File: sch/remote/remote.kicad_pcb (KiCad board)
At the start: 2 copper layers, 24 parts, among them J1 swd, J2 power_sw, J3 USB_A, Q1 DTD114E, U1 STM32F103C8Tx_usb, U2 XC6206-33, U3 TSOP17xx, Y1 8M

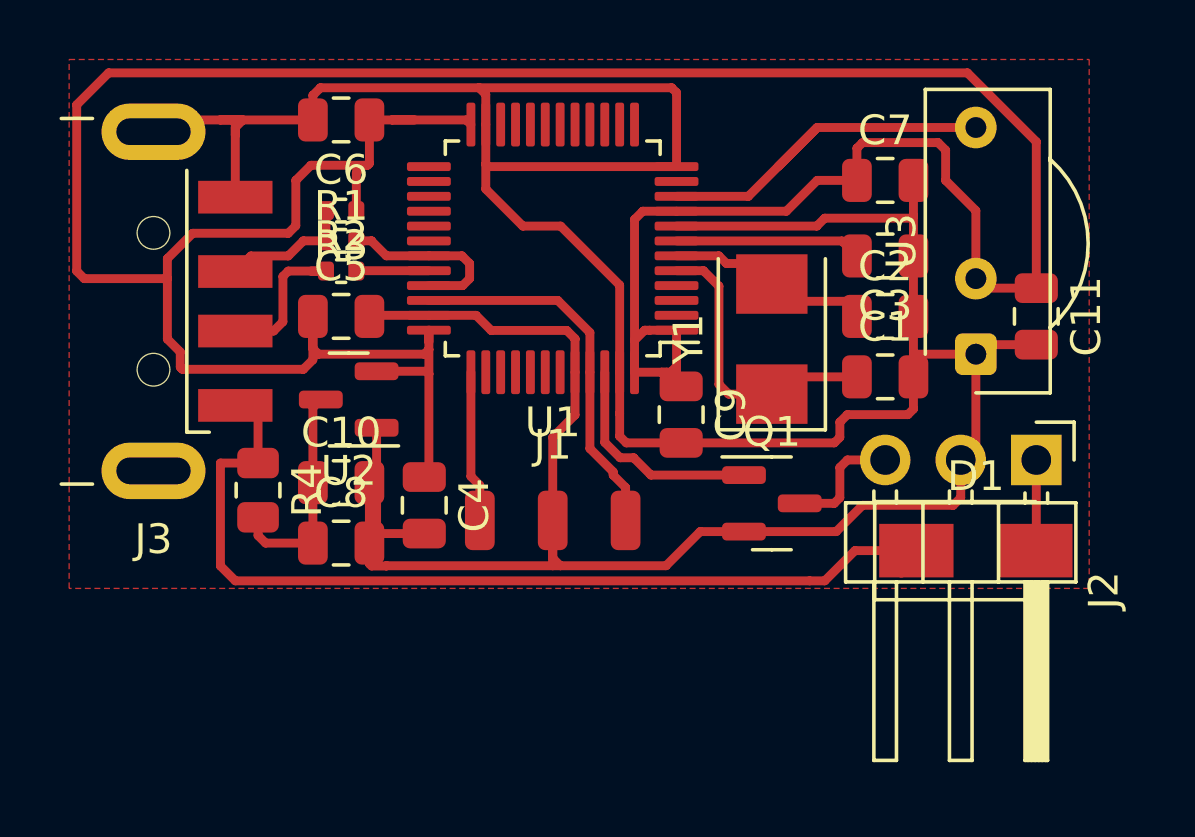
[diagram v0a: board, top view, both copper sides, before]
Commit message: 0402 caps
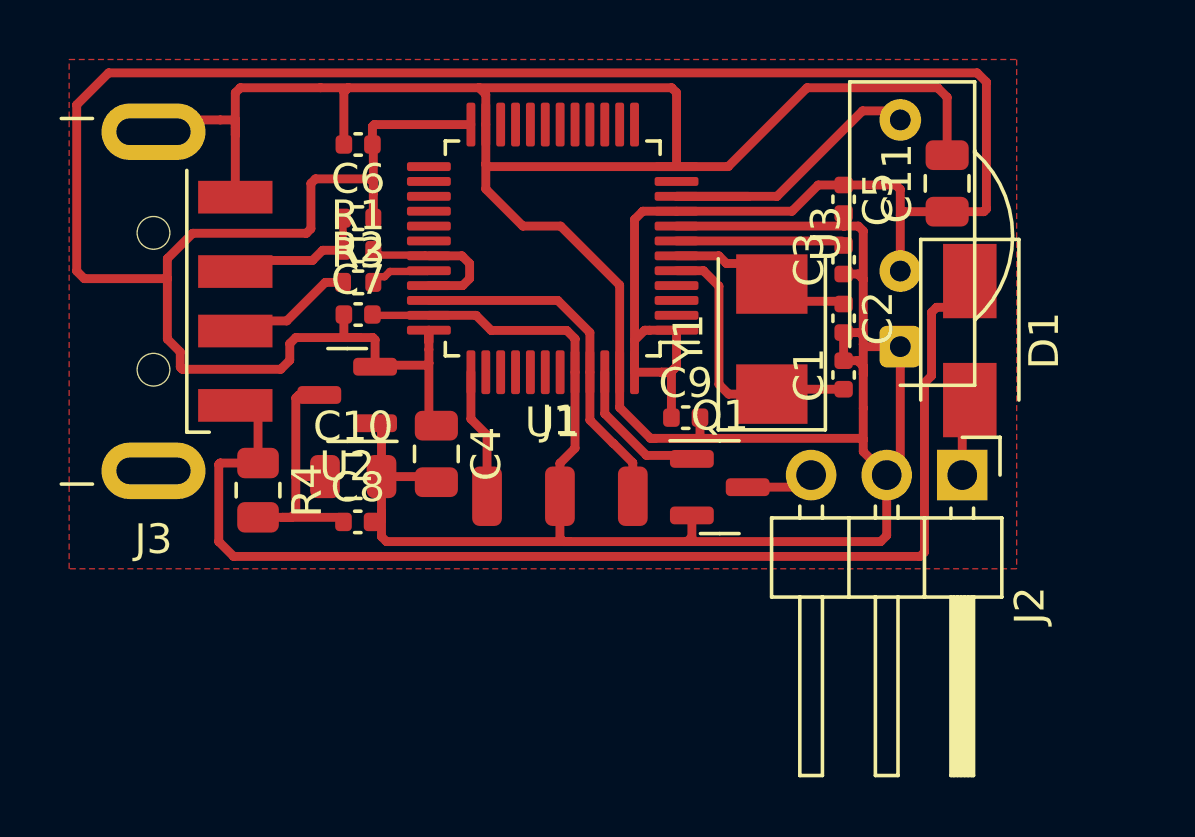
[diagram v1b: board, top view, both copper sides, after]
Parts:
- C1, C2, C3, C5, C6, C7, C8, C9: footprint Capacitor_SMD:C_0805_2012Metric -> Capacitor_SMD:C_0402_1005Metric
- moved C7 18.3 mm to (154.5, 55.6)
- moved C5 17.3 mm to (170.8, 51.7), turned to 270 degrees
- moved D1 7.06 mm to (175.1, 56.4), turned to 270 degrees
- moved C11 5.38 mm to (174.3, 51.2), turned to 90 degrees
- moved U3 2.55 mm to (172.7, 56.6)
- moved J2 2.54 mm to (174.8, 61.0)
- moved Q1 1.83 mm to (166.7, 61.4)
- moved C4 1.77 mm to (157.1, 60.2)
- moved C3 1.40 mm to (170.8, 53.7), turned to 90 degrees
- moved C1 1.40 mm to (170.8, 57.6), turned to 90 degrees
- moved C2 1.40 mm to (170.8, 55.7), turned to 270 degrees
- moved C6 1.00 mm to (154.5, 49.8)
- moved C8 0.90 mm to (154.5, 62.5)
- moved J1 0.85 mm to (161.3, 61.7)
- moved R2 0.69 mm to (154.5, 54.5)
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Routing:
- net +3V3: track 117.8 -> 104.5 mm
- net +5V: track 32.3 -> 41.3 mm
- net GND: track 134.1 -> 137.6 mm
- net /PWR: track 7.49 -> 4.95 mm
- net Net-(J2-Pad3): track 4.07 -> 2.30 mm
- net /IR: track 12.9 -> 11.1 mm
- net Net-(C10-Pad1): track 7.50 -> 9.13 mm
- net Net-(J3-Pad2): track 5.28 -> 4.35 mm
- net Net-(C3-Pad2): track 6.27 -> 5.56 mm
- net /SWCLK: track 5.11 -> 4.39 mm
- net /DP: track 6.10 -> 5.42 mm
- net Net-(C2-Pad1): track 7.02 -> 6.38 mm
- net Net-(C1-Pad1): track 9.96 -> 9.34 mm
- net Net-(D1-Pad2): track 3.06 -> 2.52 mm
- net Net-(J3-Pad3): track 4.49 -> 4.99 mm

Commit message: loger desc, new pcb for remote
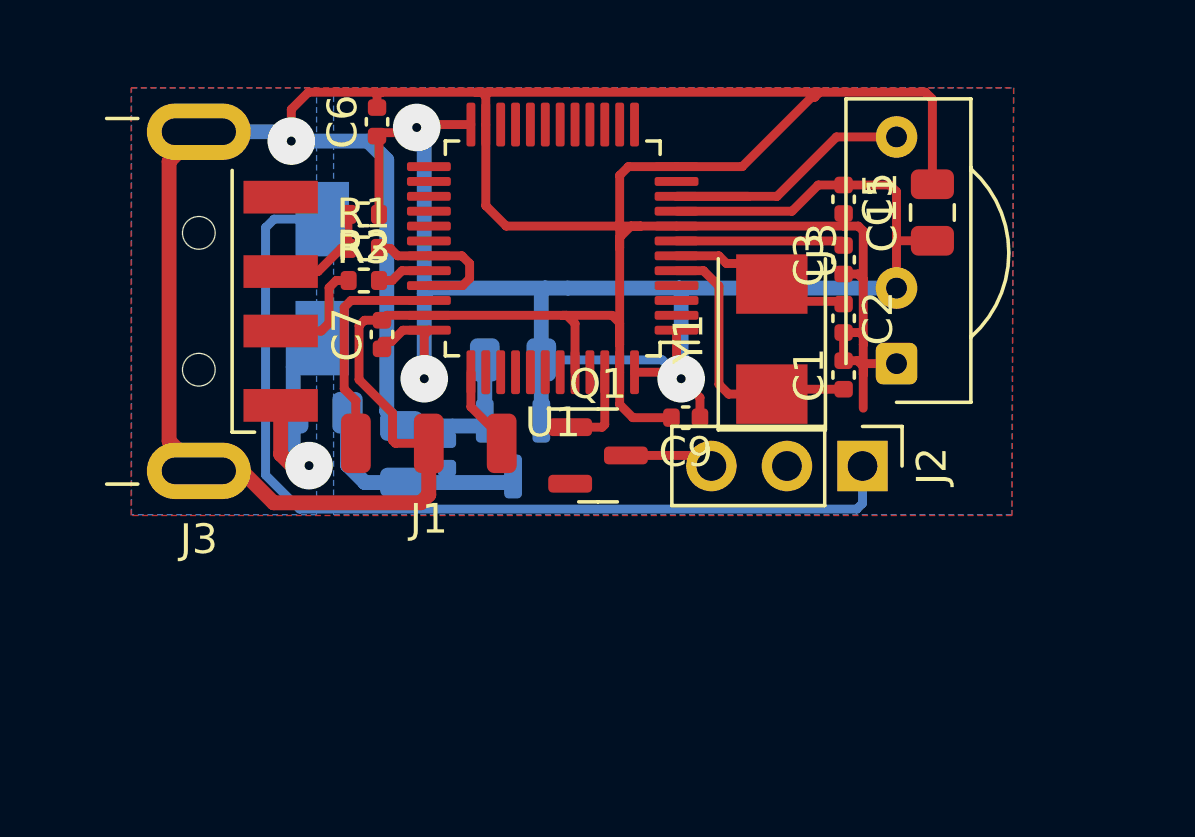
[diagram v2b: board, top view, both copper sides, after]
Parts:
- C10, C4, C8, D1, R4, U2: moved to B.Cu
- J2: footprint Connector_PinHeader_2.54mm:PinHeader_1x03_P2.54mm_Horizontal -> Connector_PinHeader_2.54mm:PinHeader_1x03_P2.54mm_Vertical
- moved D1 21.9 mm to (153.3, 54.4), turned to 90 degrees
- moved U2 5.86 mm to (159.7, 60.1), turned to 270 degrees
- moved J1 4.75 mm to (156.9, 59.9), turned to 180 degrees
- moved Q1 4.23 mm to (162.6, 60.3)
- moved C4 4.08 mm to (159.7, 57.1), turned to 180 degrees
- moved C8 3.77 mm to (157.5, 60.2), turned to 90 degrees
- moved J2 3.37 mm to (171.4, 60.7)
- moved R4 3.34 mm to (153.2, 58.9), turned to 0 degrees
- moved C10 1.79 mm to (156.0, 60.3), turned to 90 degrees
- moved J3 1.52 mm to (142.2, 55.1)
- moved C11 1.10 mm to (173.8, 52.1)
- moved C7 1.05 mm to (155.3, 56.2), turned to 90 degrees
- moved C6 0.99 mm to (155.1, 49.1), turned to 90 degrees
- moved U3 0.59 mm to (172.6, 57.2)
- moved R3 0.23 mm to (154.7, 52.2)
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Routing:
- net +3V3: track 104.5 -> 62.7 mm, vias 0 -> 3
- net +5V: track 41.3 -> 8.04 mm, vias 0 -> 1
- net Net-(D1-Pad2): track 2.52 -> 32.2 mm
- net /SWDIO: track 12.7 -> 7.68 mm
- net GND: track 137.6 -> 134.7 mm, vias 0 -> 1
- net /PWR: track 4.95 -> 2.96 mm
- net /SWCLK: track 4.39 -> 2.82 mm
- net Net-(J3-Pad3): track 4.99 -> 3.75 mm
- net Net-(C10-Pad1): track 9.13 -> 8.19 mm
- net Net-(J2-Pad3): track 2.30 -> 3.02 mm
- net Net-(J3-Pad2): track 4.35 -> 3.69 mm
- added copper zone on B.Cu, net +3V3
- added copper zone on B.Cu, net GND
